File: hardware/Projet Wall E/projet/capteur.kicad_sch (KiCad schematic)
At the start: 17 parts, among them J501 Conn_01x06, J502 Conn_01x06, J503 Conn_01x03, J504 Conn_01x06, U501 SN74AHCT1G125DBVR

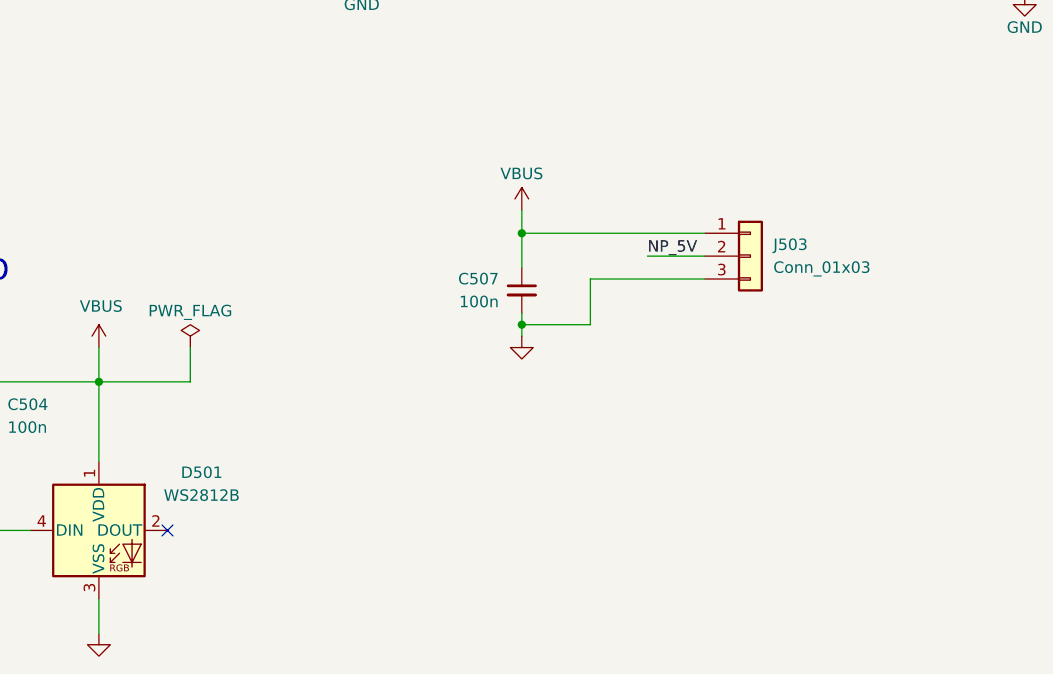
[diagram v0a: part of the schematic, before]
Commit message: verification finale effectue
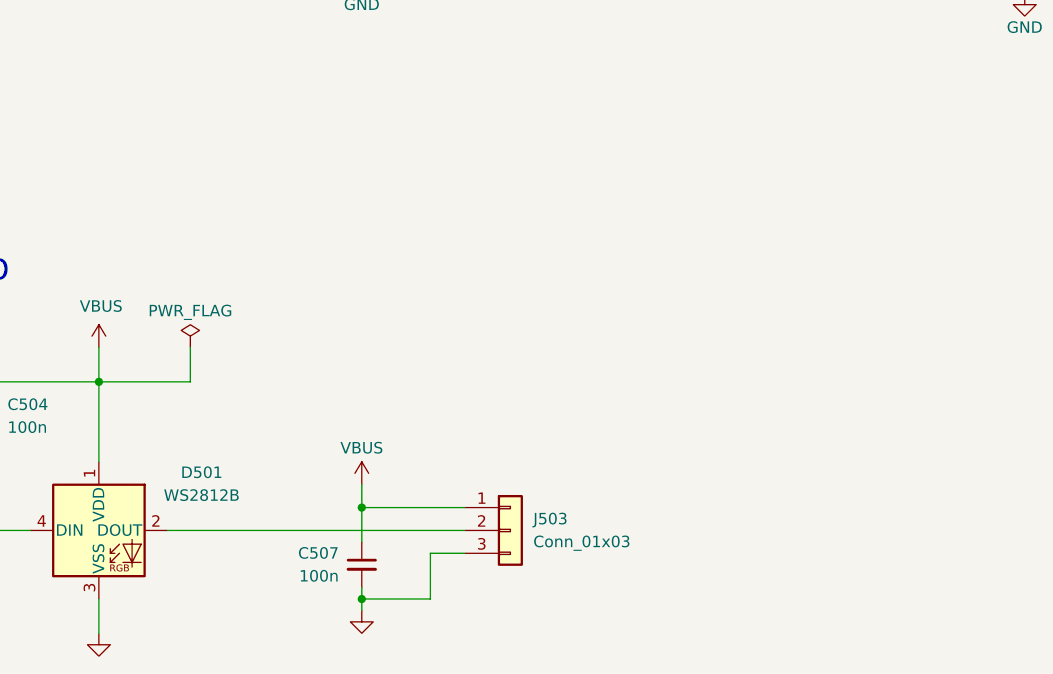
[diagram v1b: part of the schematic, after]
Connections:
- net NP_5V: no longer J503.2 (Pin_2)
- net at D501.2 (DOUT): now also J503.2 (Pin_2)
- no-connect marks 2 -> 1
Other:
- moved on the sheet: C507, J503
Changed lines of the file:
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@@
 	)
 	(junction
-		(at 130.81 140.97)
+		(at 186.69 110.49)
 		(diameter 0)
 		(color 0 0 0 0)
 	)
 	(junction
-		(at 186.69 110.49)
+		(at 113.03 171.45)
 		(diameter 0)
 		(color 0 0 0 0)
@@
 	)
 	(junction
-		(at 130.81 151.13)
+		(at 113.03 181.61)
 		(diameter 0)
 		(color 0 0 0 0)
@@
 		(at 214.63 85.09)
 	)
-	(no_connect
-		(at 91.44 173.99)
-	)
 	(wire
 		(pts
@@
 	(wire
 		(pts
+			(xy 91.44 173.99) (xy 124.46 173.99)
+		)
+		(stroke
+			(width 0)
+			(type default)
+		)
+	)
+	(wire
+		(pts
 			(xy 83.82 157.48) (xy 83.82 166.37)
 		)
@@
 	(wire
 		(pts
-			(xy 130.81 140.97) (xy 151.13 140.97)
+			(xy 113.03 171.45) (xy 124.46 171.45)
 		)
 		(stroke
@@
 	(wire
 		(pts
-			(xy 130.81 140.97) (xy 130.81 144.78)
+			(xy 113.03 171.45) (xy 113.03 175.26)
 		)
 		(stroke
@@
 	(wire
 		(pts
-			(xy 130.81 151.13) (xy 130.81 152.4)
+			(xy 113.03 181.61) (xy 113.03 182.88)
 		)
 		(stroke
@@
 	(wire
 		(pts
-			(xy 130.81 151.13) (xy 138.43 151.13)
+			(xy 113.03 181.61) (xy 120.65 181.61)
 		)
 		(stroke
@@
 	(wire
 		(pts
-			(xy 138.43 146.05) (xy 138.43 151.13)
+			(xy 120.65 176.53) (xy 120.65 181.61)
 		)
 		(stroke
@@
 	(wire
 		(pts
-			(xy 130.81 138.43) (xy 130.81 140.97)
+			(xy 113.03 168.91) (xy 113.03 171.45)
 		)
 		(stroke
@@
 	(wire
 		(pts
-			(xy 151.13 146.05) (xy 138.43 146.05)
+			(xy 124.46 176.53) (xy 120.65 176.53)
 		)
 		(stroke
@@
 	(wire
 		(pts
-			(xy 144.78 143.51) (xy 151.13 143.51)
-		)
-		(stroke
-			(width 0)
-			(type default)
-		)
-	)
-	(wire
-		(pts
 			(xy 83.82 157.48) (xy 71.12 157.48)
 		)
@@
 	(wire
 		(pts
-			(xy 130.81 149.86) (xy 130.81 151.13)
+			(xy 113.03 180.34) (xy 113.03 181.61)
 		)
 		(stroke
@@
 		)
 	)
-	(label "NP_5V"
-		(at 144.78 143.51 0)
-		(effects
-			(font
-				(size 1.27 1.27)
-			)
-			(justify left bottom)
-		)
-	)
 	(label "SDA_CAPT"
 		(at 207.01 92.71 180)
@@
 	(symbol
 		(lib_id "Connector_Generic:Conn_01x03")
-		(at 156.21 143.51 0)
+		(at 129.54 173.99 0)
 		(unit 1)
 		(body_style 1)
@@
 		(fields_autoplaced yes)
 		(property "Reference" "J503"
-			(at 158.75 142.2399 0)
+			(at 132.08 172.7199 0)
 			(show_name no)
 			(do_not_autoplace no)
@@
 		)
 		(property "Value" "Conn_01x03"
-			(at 158.75 144.7799 0)
+			(at 132.08 175.2599 0)
 			(show_name no)
 			(do_not_autoplace no)
@@
 		)
 		(property "Footprint" "Connector_PinHeader_2.54mm:PinHeader_1x03_P2.54mm_Vertical"
-			(at 156.21 143.51 0)
+			(at 129.54 173.99 0)
 			(hide yes)
 			(show_name no)
@@
 		)
 		(property "Datasheet" ""
-			(at 156.21 143.51 0)
+			(at 129.54 173.99 0)
 			(hide yes)
 			(show_name no)
@@
 		)
 		(property "Description" "Generic connector, single row, 01x03, script generated (kicad-library-utils/schlib/autogen/connector/)"
-			(at 156.21 143.51 0)
+			(at 129.54 173.99 0)
 			(hide yes)
 			(show_name no)
@@
 		)
 		(property "JLCPCB Part#" "C49257"
-			(at 156.21 143.51 0)
+			(at 129.54 173.99 0)
 			(hide yes)
 			(show_name no)
@@
 		)
 		(property "KLC_S3.3" ""
-			(at 156.21 143.51 0)
+			(at 129.54 173.99 0)
 			(hide yes)
 			(show_name no)
@@
 		)
 		(property "KLC_S4.1" ""
-			(at 156.21 143.51 0)
+			(at 129.54 173.99 0)
 			(hide yes)
 			(show_name no)
@@
 		)
 		(property "Sim.Device" ""
-			(at 156.21 143.51 0)
+			(at 129.54 173.99 0)
 			(hide yes)
 			(show_name no)
@@
 	(symbol
 		(lib_id "power:+5V")
-		(at 130.81 138.43 0)
+		(at 113.03 168.91 0)
 		(unit 1)
 		(body_style 1)
@@
 		(dnp no)
 		(property "Reference" "#PWR0513"
-			(at 130.81 142.24 0)
+			(at 113.03 172.72 0)
 			(hide yes)
 			(show_name no)
@@
 		)
 		(property "Value" "VBUS"
-			(at 130.81 134.366 0)
+			(at 113.03 164.846 0)
 			(show_name no)
 			(do_not_autoplace no)
@@
 		)
 		(property "Footprint" ""
-			(at 130.81 138.43 0)
+			(at 113.03 168.91 0)
 			(hide yes)
 			(show_name no)
@@
 		)
 		(property "Datasheet" ""
-			(at 130.81 138.43 0)
+			(at 113.03 168.91 0)
 			(hide yes)
 			(show_name no)
@@
 		)
 		(property "Description" "Power symbol creates a global label with name \"+5V\""
-			(at 130.81 138.43 0)
+			(at 113.03 168.91 0)
 			(hide yes)
 			(show_name no)
@@
 	(symbol
 		(lib_id "power:GND")
-		(at 130.81 152.4 0)
+		(at 113.03 182.88 0)
 		(unit 1)
 		(body_style 1)
@@
 		(fields_autoplaced yes)
 		(property "Reference" "#PWR0514"
-			(at 130.81 158.75 0)
+			(at 113.03 189.23 0)
 			(hide yes)
 			(show_name no)
@@
 		)
 		(property "Value" "GND"
-			(at 130.81 157.48 0)
+			(at 113.03 187.96 0)
 			(hide yes)
 			(show_name no)
@@
 		)
 		(property "Footprint" ""
-			(at 130.81 152.4 0)
+			(at 113.03 182.88 0)
 			(hide yes)
 			(show_name no)
@@
 		)
 		(property "Datasheet" ""
-			(at 130.81 152.4 0)
+			(at 113.03 182.88 0)
 			(hide yes)
 			(show_name no)
@@
 		)
 		(property "Description" "Power symbol creates a global label with name \"GND\" , ground"
-			(at 130.81 152.4 0)
+			(at 113.03 182.88 0)
 			(hide yes)
 			(show_name no)
@@
 	(symbol
 		(lib_id "Device:C_Small")
-		(at 130.81 147.32 0)
+		(at 113.03 177.8 0)
 		(mirror y)
 		(unit 1)
@@
 		(dnp no)
 		(property "Reference" "C507"
-			(at 128.27 146.0562 0)
+			(at 110.49 176.5362 0)
 			(show_name no)
 			(do_not_autoplace no)
@@
 		)
 		(property "Value" "100n"
-			(at 128.27 148.5962 0)
+			(at 110.49 179.0762 0)
 			(show_name no)
 			(do_not_autoplace no)
@@
 		)
 		(property "Footprint" "Capacitor_SMD:C_0402_1005Metric"
-			(at 130.81 147.32 0)
+			(at 113.03 177.8 0)
 			(hide yes)
 			(show_name no)
@@
 		)
 		(property "Datasheet" ""
-			(at 130.81 147.32 0)
+			(at 113.03 177.8 0)
 			(hide yes)
 			(show_name no)
@@
 		)
 		(property "Description" "Unpolarized capacitor, small symbol"
-			(at 130.81 147.32 0)
+			(at 113.03 177.8 0)
 			(hide yes)
 			(show_name no)
@@
 		)
 		(property "JLCPCB Part #" ""
-			(at 130.81 147.32 0)
+			(at 113.03 177.8 0)
 			(hide yes)
 			(show_name no)
@@
 		)
 		(property "JLCPCB Part#" "C1525"
-			(at 130.81 147.32 0)
+			(at 113.03 177.8 0)
 			(hide yes)
 			(show_name no)
@@
 		)
 		(property "Sim.Device" ""
-			(at 130.81 147.32 0)
+			(at 113.03 177.8 0)
 			(hide yes)
 			(show_name no)
